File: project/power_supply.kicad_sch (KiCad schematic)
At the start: 17 parts, among them J1 USB_C_Receptacle_USB2.0_16P, U1 USBLC6-2SC6, U2 MIC5356-S4YMME

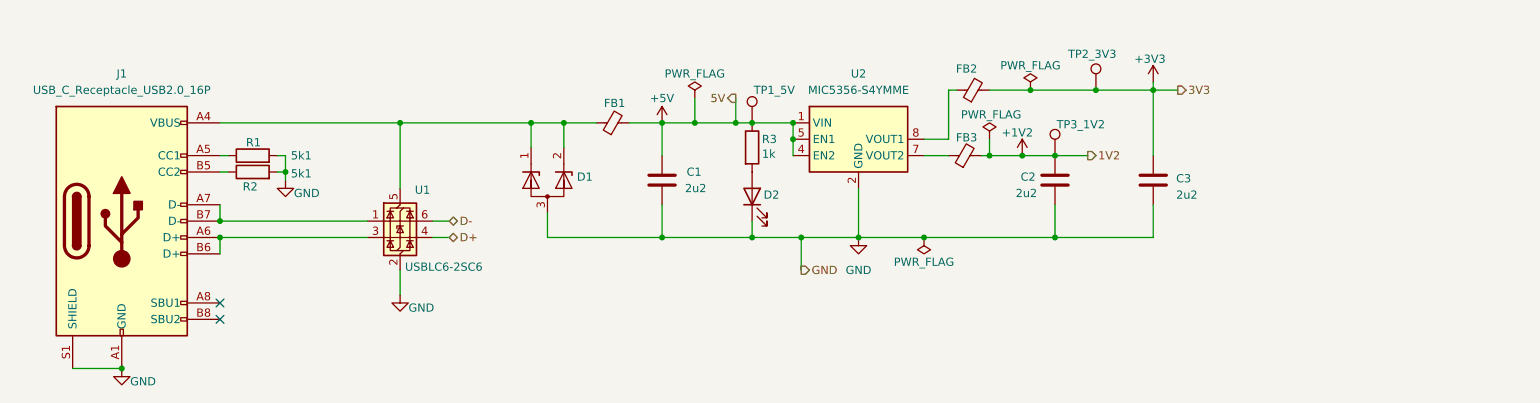
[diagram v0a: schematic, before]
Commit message: Guardado previo, FTDI casi listo
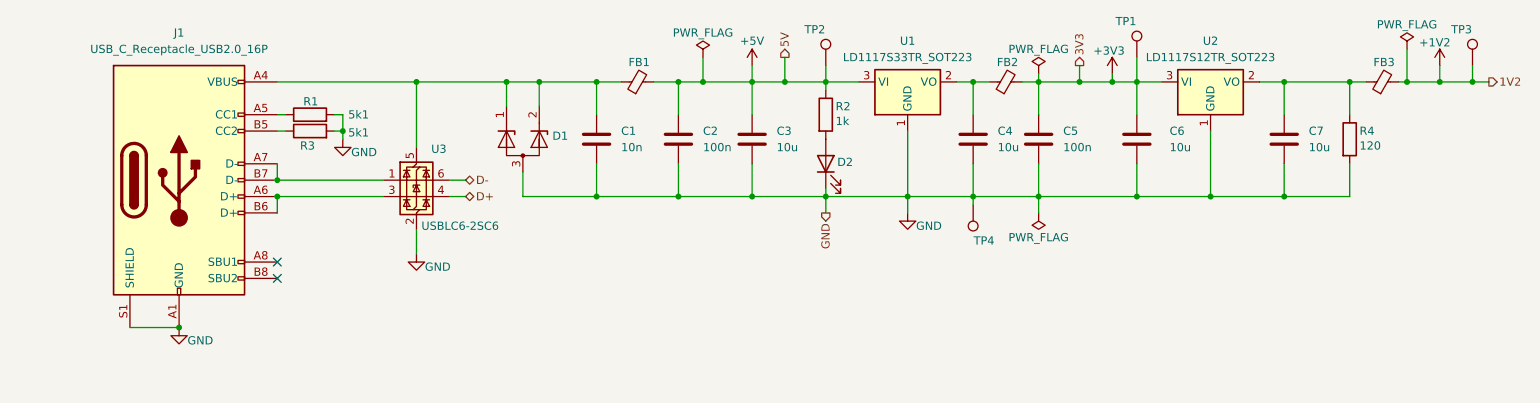
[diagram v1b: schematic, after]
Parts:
- removed TP1_5V, TP2_3V3, TP3_1V2: TestPoint, symbol Connector:TestPoint
- removed U1: USBLC6-2SC6, Package_TO_SOT_SMD:SOT-23-6, symbol Power_Protection:USBLC6-2SC6
- removed U2: MIC5356-S4YMME, Package_SO:MSOP-8-1EP_3x3mm_P0.65mm_EP2.5x3mm_Mask1.73x2.36mm_ThermalVias, symbol Regulator_Linear:MIC5356-S4YMME
- added C4, C6, C7: 10u, symbol Device:C
- added C5: 100n, symbol Device:C
- added R4: 120, symbol Device:R
- added TP1: TP2_3V1, symbol Connector:TestPoint
- added TP2: TP1_5V1, symbol Connector:TestPoint
- added TP3: TP3_1V2, symbol Connector:TestPoint
- added TP4: TP4_GND, symbol Connector:TestPoint
- added U1: LD1117S33TR_SOT223, Package_TO_SOT_SMD:SOT-223-3_TabPin2, symbol Regulator_Linear:LD1117S33TR_SOT223
- added U2: LD1117S12TR_SOT223, Package_TO_SOT_SMD:SOT-223-3_TabPin2, symbol Regulator_Linear:LD1117S12TR_SOT223
- added U3: USBLC6-2SC6, Package_TO_SOT_SMD:SOT-23-6, symbol Power_Protection:USBLC6-2SC6
- C1: value 2u2 -> 10n
- C2: value 2u2 -> 100n
- C3: value 2u2 -> 10u
- R2: value 5k1 -> 1k
- R3: value 1k -> 5k1
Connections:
- net +1V2: now also TP3.1; no longer C2.1
- net +3V3: now also C5.1, C6.1, TP1.1, U2.3 (VI); no longer C3.1
- net +5V: now also C2.1, C3.1, R2.1, TP2.1, U1.3 (VI); no longer C1.1, R3.1
- net D+: now also U3.4 (I/O2)
- net D-: now also U3.6 (I/O1)
- net GND: now also R3.2, C4.2, C5.2, C6.2, C7.2, R4.2, TP4.1, U1.1 (GND), U2.1 (GND), U3.2 (GND); no longer R2.2
- net at D1.1 (K), D1.2 (K), FB1.1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: now also C1.1, U3.5 (VBUS)
- net at D2.2 (A): now also R2.2; no longer R3.2
- net at FB3.1: now also C7.1, R4.1, U2.2 (VO)
- net at FB2.1: now also C4.1, U1.2 (VO)
- net at J1.A6 (D+), J1.B6 (D+): now also U3.3 (I/O2)
- net at J1.A7 (D-), J1.B7 (D-): now also U3.1 (I/O1)
- net at J1.B5 (CC2): now also R3.1; no longer R2.1
